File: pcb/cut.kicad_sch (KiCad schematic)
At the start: 42 parts, among them J4 RJ12, J5 RJ12, J6 MV132, J7 MV132, K1 AZ850-5, K2 AZ850-5, Q1 2N7002, Q2 2N7002, U5 PC817, U6 PC817

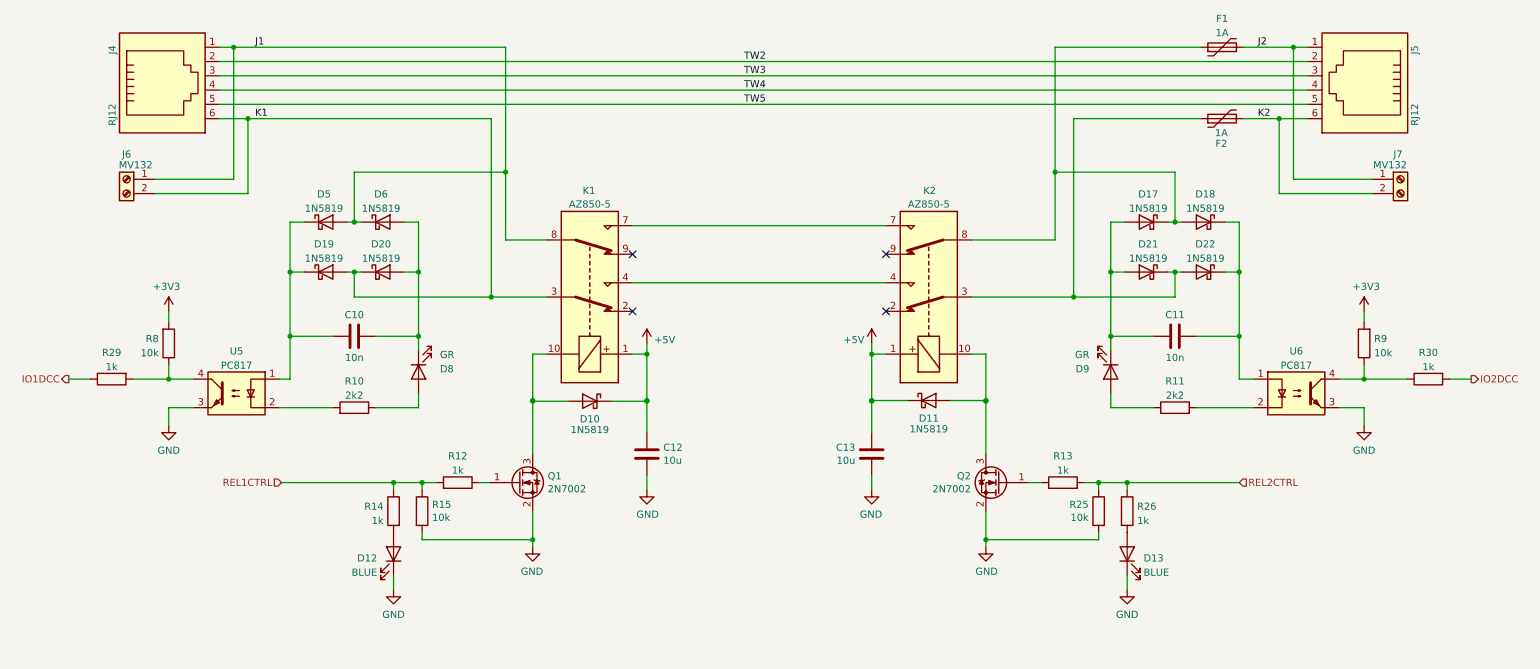
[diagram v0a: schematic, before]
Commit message: Add separate resistors for LEDs.
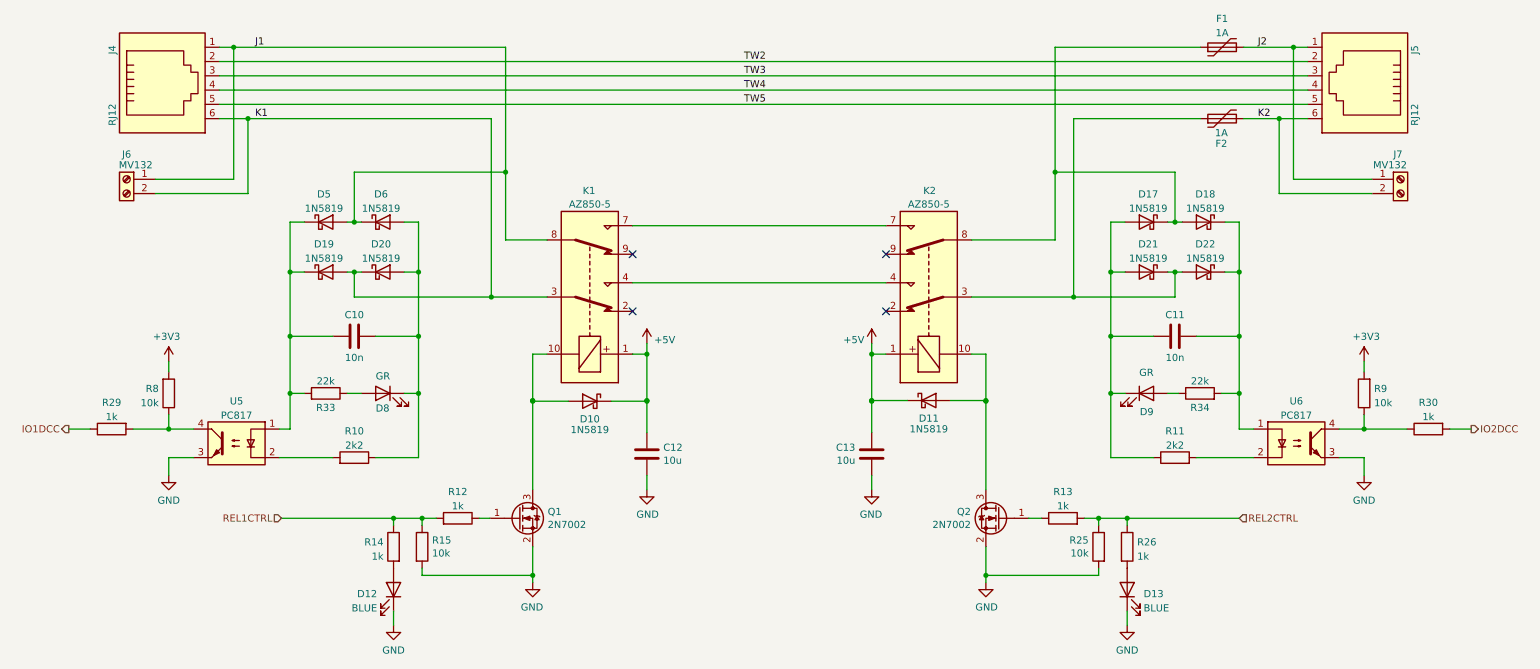
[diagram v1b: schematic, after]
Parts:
- added R33, R34: 22k, Resistor_SMD:R_0805_2012Metric, symbol Device:R
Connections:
- net at C11.1, D17.2 (A), D21.2 (A)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: now also R11.1
- net at D9.2 (A): now also R34.1; no longer R11.1
- net at C10.2, D20.2 (A), D6.2 (A)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: now also R10.1
- net at C10.1, D19.1 (K), D5.1 (K)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: now also R33.2
- net at D8.2 (A): now also R33.1; no longer R10.1
- net at C11.2, D18.1 (K), D22.1 (K)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: now also R34.2
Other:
- moved on the sheet: D12, D13, D8, D9, Q1, Q2, R10, R11, R12, R13, R14, R15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
